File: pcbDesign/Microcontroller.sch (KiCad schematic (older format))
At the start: 8 parts, among them U2 ATSAME51J18A-A, Y1 32.768

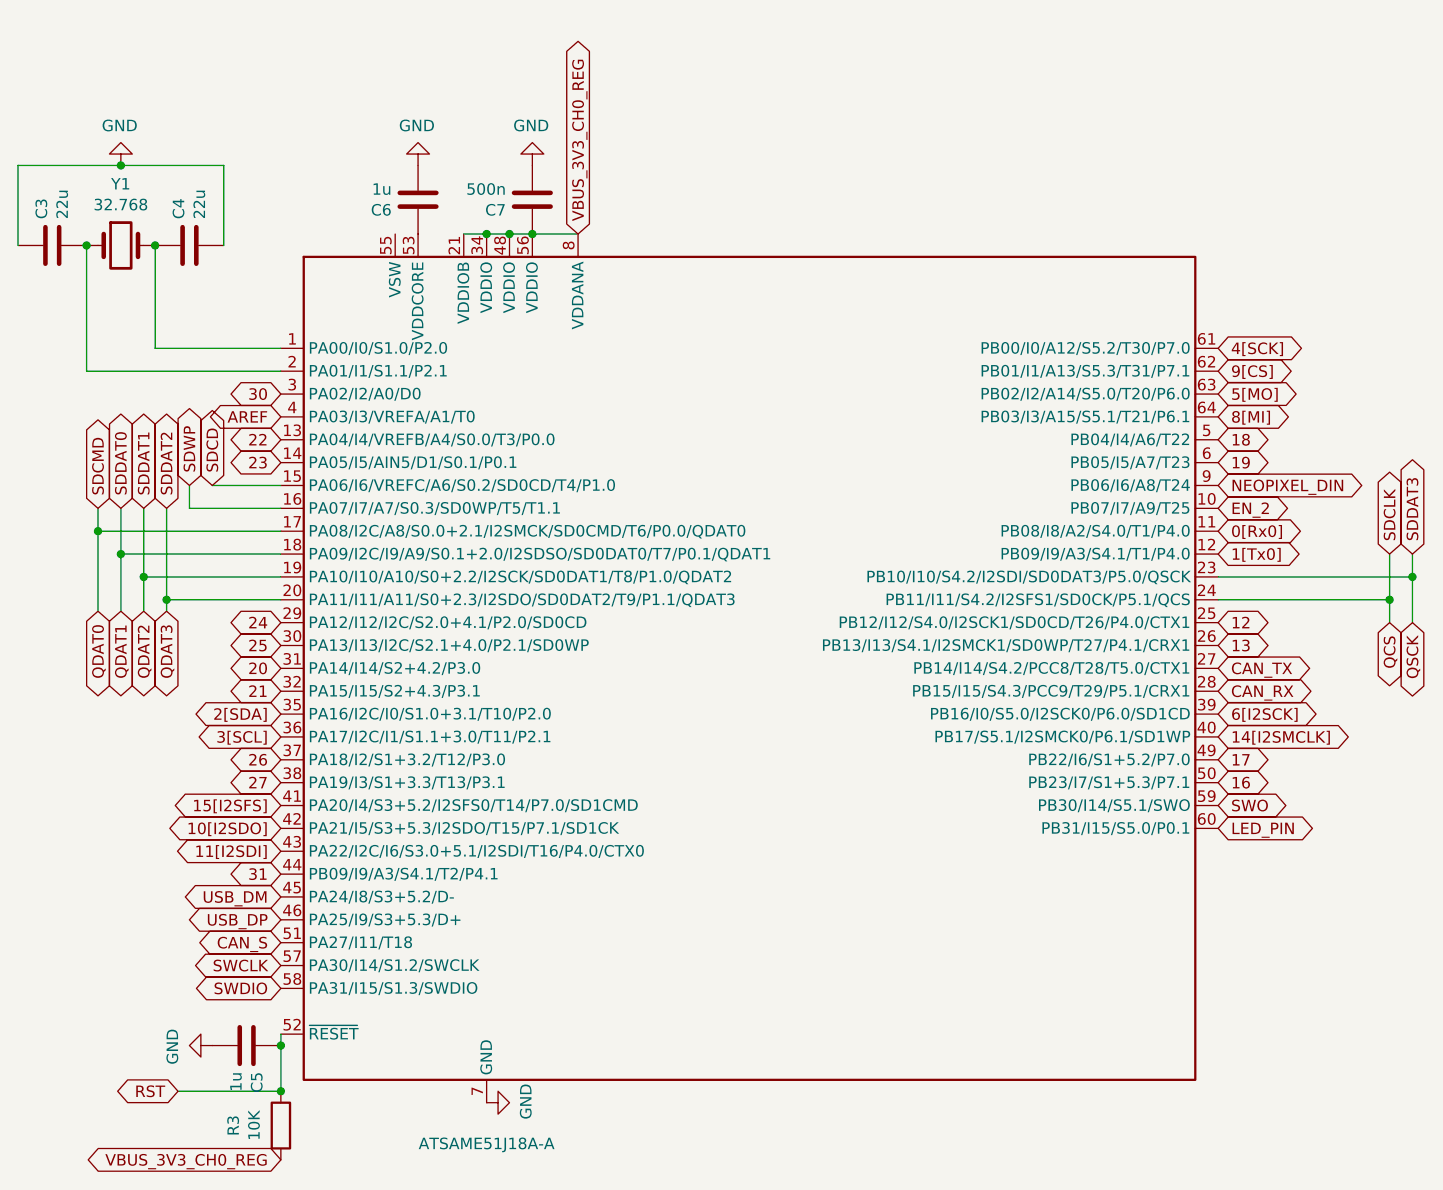
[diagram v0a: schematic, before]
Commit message: Finnished routing
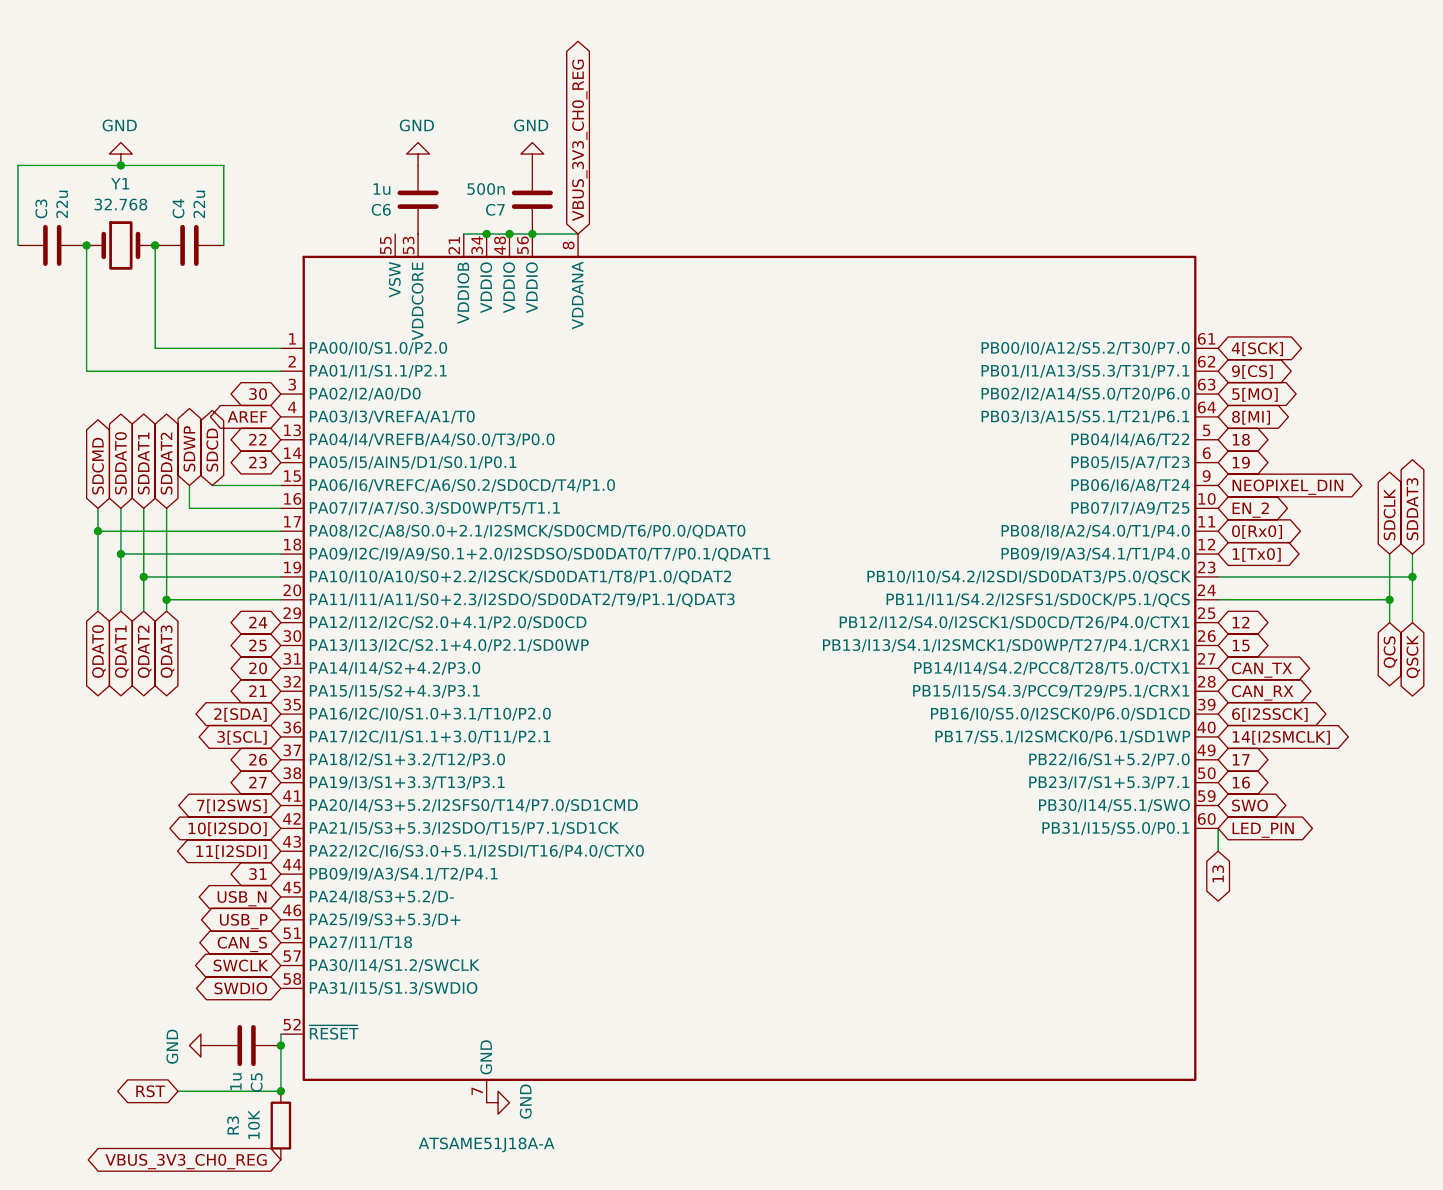
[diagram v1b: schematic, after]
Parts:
- Y1: footprint Oscillator:Oscillator_SMD_Abracon_ASCO-4Pin_1.6x1.2mm -> Crystal:Crystal_SMD_2012-2Pin_2.0x1.2mm
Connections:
- net LED_PIN is gone; now on net 13: U2.60 (PB31/I15/S5.0/P0.1)
- net 13: no longer U2.26 (PB13/I13/S4.1/I2SMCK1/SD0WP/T27/P4.1/CRX1)
- net 15[I2SFS] renamed 7[I2SWS]
- net 6[I2SCK] renamed 6[I2SSCK]
- net USB_DM renamed USB_N
- net USB_DP renamed USB_P
- new net 15: U2.26 (PB13/I13/S4.1/I2SMCK1/SD0WP/T27/P4.1/CRX1)
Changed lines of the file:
@@
 $EndComp
 Text GLabel 4400 4800 0    50   BiDi ~ 0
-USB_DM
+USB_N
 Text GLabel 4400 4900 0    50   BiDi ~ 0
-USB_DP
+USB_P
 Wire Wire Line
 	4400 5400 4400 5450
@@
 AREF
 Text GLabel 8500 4000 2    50   BiDi ~ 0
-6[I2SCK]
+6[I2SSCK]
 Text GLabel 8500 4100 2    50   BiDi ~ 0
 14[I2SMCLK]
@@
 10[I2SDO]
 Text GLabel 4400 4400 0    50   BiDi ~ 0
-15[I2SFS]
+7[I2SWS]
 Text GLabel 3950 5650 0    50   BiDi ~ 0
 RST
@@
 Text GLabel 8500 3600 2    50   BiDi ~ 0
 12
-Text GLabel 8500 3700 2    50   BiDi ~ 0
+Text GLabel 8500 4600 3    50   BiDi ~ 0
 13
 Text GLabel 4400 2800 0    50   BiDi ~ 0
@@
 F 0 "Y1" H 3700 2218 50  0000 C CNN
 F 1 "32.768" H 3700 2127 50  0000 C CNN
-F 2 "Oscillator:Oscillator_SMD_Abracon_ASCO-4Pin_1.6x1.2mm" H 3700 1950 50  0001 C CNN
+F 2 "Crystal:Crystal_SMD_2012-2Pin_2.0x1.2mm" H 3700 1950 50  0001 C CNN
 F 3 "~" H 3700 1950 50  0001 C CNN
 	1    3700 1950
@@
 	-1   0    0    1
 $EndComp
+Wire Wire Line
+	8500 4600 8500 4500
+Text GLabel 8500 3700 2    50   BiDi ~ 0
+15
 $EndSCHEMATC
